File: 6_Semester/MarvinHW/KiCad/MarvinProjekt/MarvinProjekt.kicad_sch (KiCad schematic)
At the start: 30 parts, among them J1 Conn_02x03_Odd_Even, J2 Conn_01x04_Pin, SW1 Reset, SW2 Boot, SW3 Volume+, SW4 Volume-, SW5 Modi1, SW6 Modi0, SW8 Reset, SW9 Boot, U1 ESP32-S3-WROOM-1, U10 ToF, U9 WS2812, X1 USB3.1C16PFSMT

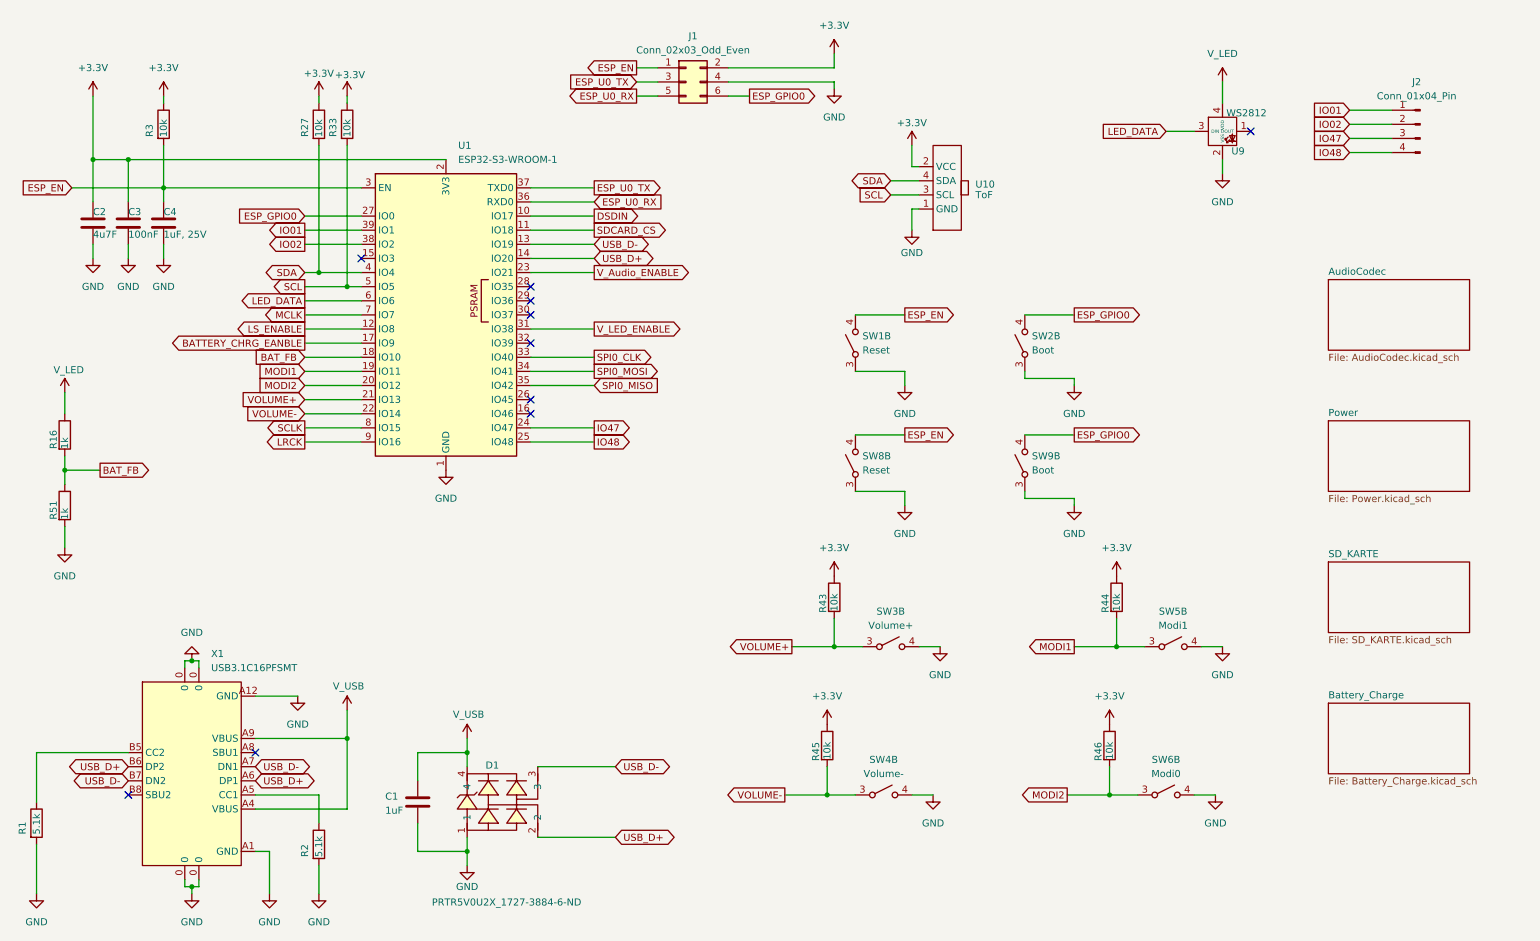
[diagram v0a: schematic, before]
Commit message: Finished Layout
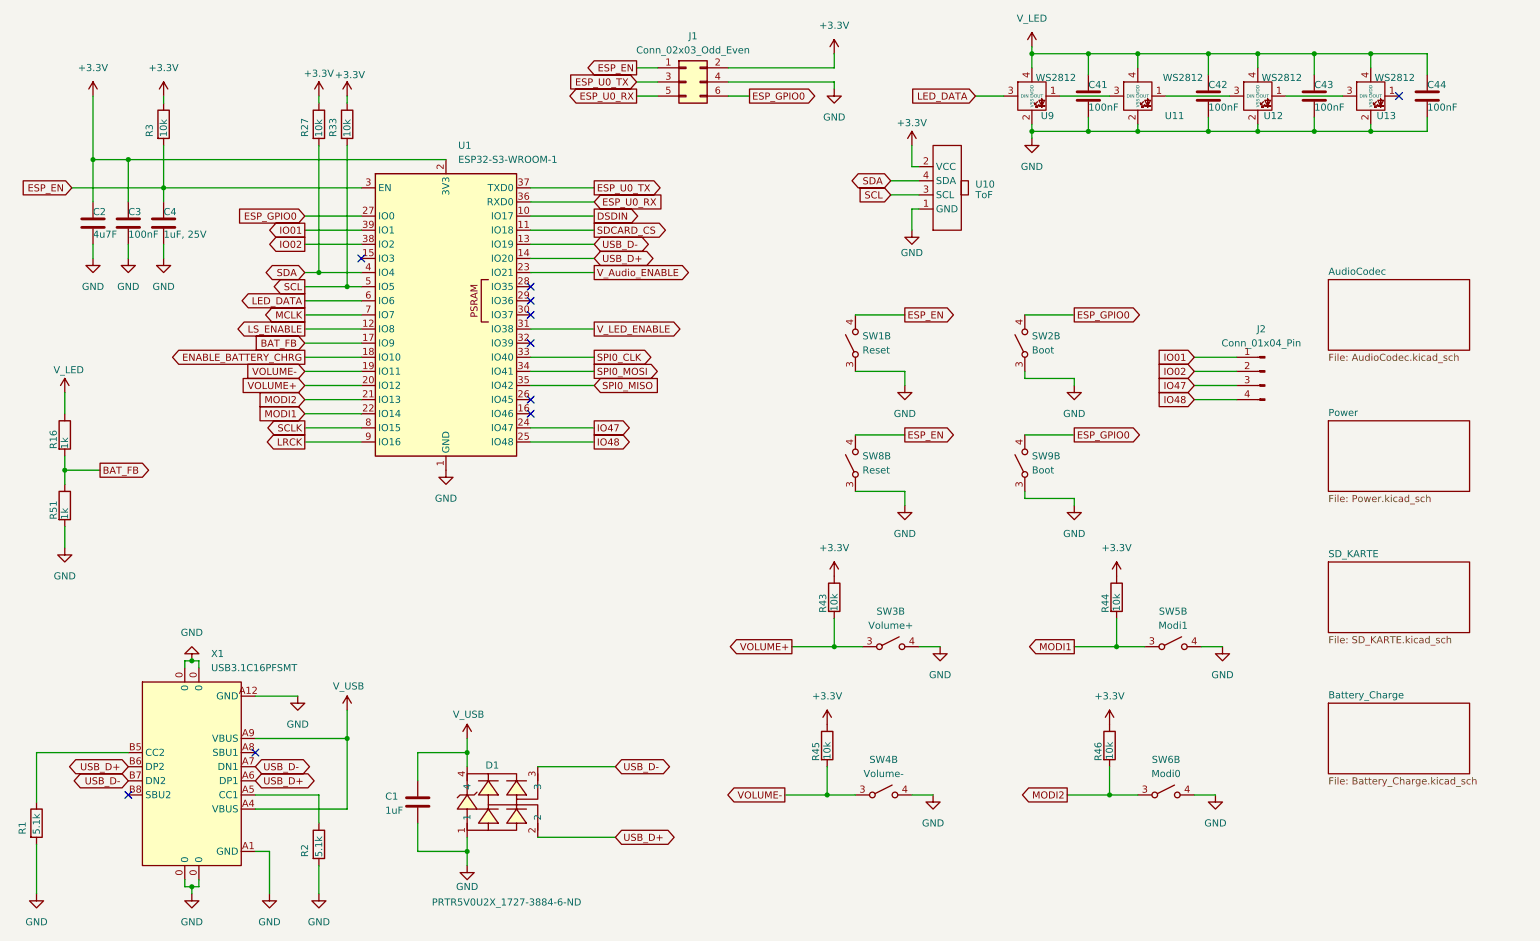
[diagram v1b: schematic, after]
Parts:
- added C41, C42, C43, C44: 100nF, Capacitor_SMD:C_0805_2012Metric_Pad1.18x1.45mm_HandSolder, symbol Device:C
- added U11, U12, U13: WS2812, LED_SMD:LED_WS2812B-2020_PLCC4_2.0x2.0mm, symbol Library:WS2812
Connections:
- net BATTERY_CHRG_EANBLE is gone; now on net BAT_FB: U1.17 (IO9)
- net BAT_FB: no longer U1.18 (IO10)
- net GND: now also C41.2, C42.2, C43.2, C44.2, U11.2 (VSS), U12.2 (VSS), U13.2 (VSS)
- net MODI1: now also U1.22 (IO14); no longer U1.19 (IO11)
- net MODI2: now also U1.21 (IO13); no longer U1.20 (IO12)
- net VOLUME+: now also U1.20 (IO12); no longer U1.21 (IO13)
- net VOLUME-: now also U1.19 (IO11); no longer U1.22 (IO14)
- net V_LED: now also C41.1, C42.1, C43.1, C44.1, U11.4 (VDD), U12.4 (VDD), U13.4 (VDD)
- net at U9.1 (DOUT): now also U11.3 (DIN)
- new net: U12.1 (DOUT), U13.3 (DIN)
- new net: U11.1 (DOUT), U12.3 (DIN)
- new net ENABLE_BATTERY_CHRG: U1.18 (IO10)
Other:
- moved on the sheet: J2, U9
